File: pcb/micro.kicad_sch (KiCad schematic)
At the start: 23 parts, among them SW1 SW_Nidec_CAS-120A1, U1 ESP32-C6, Y1 7M40000049

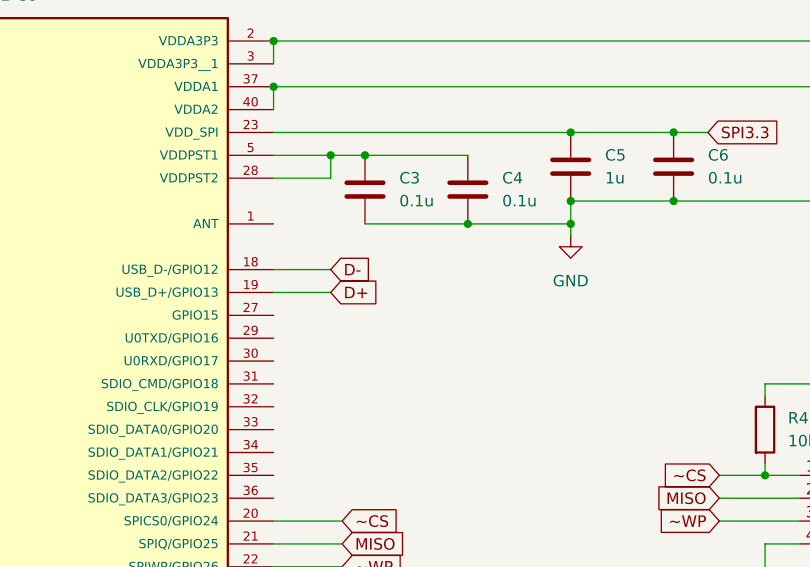
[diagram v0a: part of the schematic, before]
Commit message: Schematic finalized and general layout completed
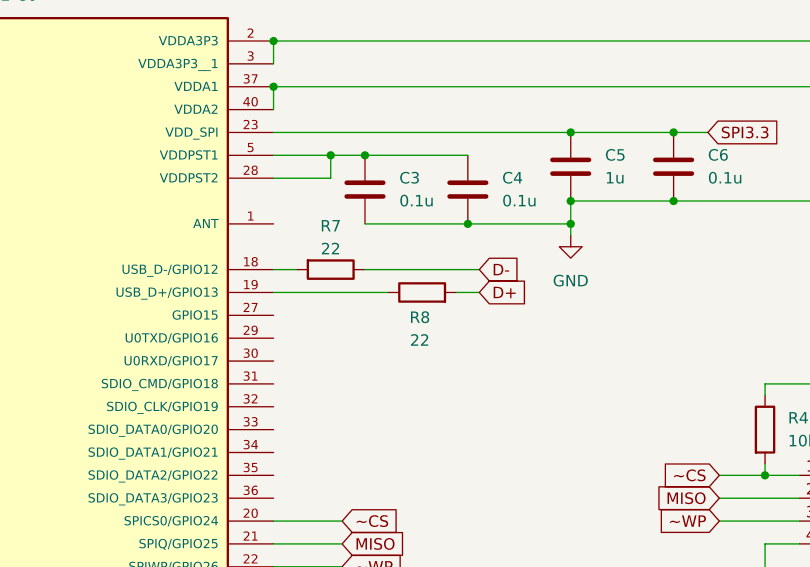
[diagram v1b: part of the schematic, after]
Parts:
- added R7, R8: 22, Resistor_SMD:R_0402_1005Metric_Pad0.72x0.64mm_HandSolder, symbol Device:R
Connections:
- net D+: now also R8.2; no longer U1.19 (USB_D+/GPIO13)
- net D-: now also R7.1; no longer U1.18 (USB_D-/GPIO12)
- new net: R7.2, U1.18 (USB_D-/GPIO12)
- new net: R8.1, U1.19 (USB_D+/GPIO13)
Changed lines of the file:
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@@
 	(wire
 		(pts
-			(xy 142.24 87.63) (xy 148.59 87.63)
+			(xy 162.56 90.17) (xy 165.1 90.17)
 		)
 		(stroke
@@
 	(wire
 		(pts
+			(xy 142.24 87.63) (xy 144.78 87.63)
+		)
+		(stroke
+			(width 0)
+			(type default)
+		)
+	)
+	(wire
+		(pts
 			(xy 54.61 115.57) (xy 54.61 120.65)
 		)
@@
 	(wire
 		(pts
-			(xy 142.24 90.17) (xy 148.59 90.17)
-		)
-		(stroke
-			(width 0)
-			(type default)
-		)
-	)
-	(wire
-		(pts
 			(xy 113.03 176.53) (xy 97.79 176.53)
 		)
@@
 	(wire
 		(pts
+			(xy 142.24 90.17) (xy 154.94 90.17)
+		)
+		(stroke
+			(width 0)
+			(type default)
+		)
+	)
+	(wire
+		(pts
 			(xy 142.24 62.23) (xy 142.24 64.77)
 		)
@@
 	(wire
 		(pts
+			(xy 152.4 87.63) (xy 165.1 87.63)
+		)
+		(stroke
+			(width 0)
+			(type default)
+		)
+	)
+	(wire
+		(pts
 			(xy 76.2 85.09) (xy 81.28 85.09)
 		)
@@
 	(global_label "D+"
 		(shape input)
-		(at 148.59 90.17 0)
+		(at 165.1 90.17 0)
 		(fields_autoplaced yes)
 		(effects
@@
 		)
 		(property "Intersheetrefs" "${INTERSHEET_REFS}"
-			(at 154.4176 90.17 0)
+			(at 170.9276 90.17 0)
 			(effects
 				(font
@@
 	(global_label "D-"
 		(shape input)
-		(at 148.59 87.63 0)
+		(at 165.1 87.63 0)
 		(fields_autoplaced yes)
 		(effects
@@
 		)
 		(property "Intersheetrefs" "${INTERSHEET_REFS}"
-			(at 154.4176 87.63 0)
+			(at 170.9276 87.63 0)
 			(effects
 				(font
@@
 	)
 	(symbol
+		(lib_id "Device:R")
+		(at 148.59 87.63 270)
+		(unit 1)
+		(exclude_from_sim no)
+		(in_bom yes)
+		(on_board yes)
+		(dnp no)
+		(property "Reference" "R7"
+			(at 148.59 82.804 90)
+			(effects
+				(font
+					(size 1.27 1.27)
+				)
+			)
+		)
+		(property "Value" "22"
+			(at 148.59 85.344 90)
+			(effects
+				(font
+					(size 1.27 1.27)
+				)
+			)
+		)
+		(property "Footprint" "Resistor_SMD:R_0402_1005Metric_Pad0.72x0.64mm_HandSolder"
+			(at 148.59 85.852 90)
+			(effects
+				(font
+					(size 1.27 1.27)
+				)
+				(hide yes)
+			)
+		)
+		(property "Datasheet" "~"
+			(at 148.59 87.63 0)
+			(effects
+				(font
+					(size 1.27 1.27)
+				)
+				(hide yes)
+			)
+		)
+		(property "Description" "Resistor"
+			(at 148.59 87.63 0)
+			(effects
+				(font
+					(size 1.27 1.27)
+				)
+				(hide yes)
+			)
+		)
+		(pin "2"
+		)
+		(pin "1"
+		)
+		(instances
+			(project "60_keyboard"
+				(path "/60f4ab9d-718b-428d-904c-5042759d3860/a5dc5d45-cfa6-4235-a666-1339e0663470"
+					(reference "R7")
+					(unit 1)
+				)
+			)
+		)
+	)
+	(symbol
 		(lib_id "Device:C")
 		(at 259.08 66.04 0)
@@
 					(unit 1)
 				)
+			)
+		)
+	)
+	(symbol
+		(lib_id "Device:R")
+		(at 158.75 90.17 90)
+		(unit 1)
+		(exclude_from_sim no)
+		(in_bom yes)
+		(on_board yes)
+		(dnp no)
+		(property "Reference" "R8"
+			(at 158.496 92.964 90)
+			(effects
+				(font
+					(size 1.27 1.27)
+				)
+			)
+		)
+		(property "Value" "22"
+			(at 158.496 95.504 90)
+			(effects
+				(font
+					(size 1.27 1.27)
+				)
+			)
+		)
+		(property "Footprint" "Resistor_SMD:R_0402_1005Metric_Pad0.72x0.64mm_HandSolder"
+			(at 158.75 91.948 90)
+			(effects
+				(font
+					(size 1.27 1.27)
+				)
+				(hide yes)
+			)
+		)
+		(property "Datasheet" "~"
+			(at 158.75 90.17 0)
+			(effects
+				(font
+					(size 1.27 1.27)
+				)
+				(hide yes)
+			)
+		)
+		(property "Description" "Resistor"
+			(at 158.75 90.17 0)
+			(effects
+				(font
+					(size 1.27 1.27)
+				)
+				(hide yes)
+			)
+		)
+		(pin "2"
+		)
+		(pin "1"
+		)
+		(instances
+			(project "60_keyboard"
+				(path "/60f4ab9d-718b-428d-904c-5042759d3860/a5dc5d45-cfa6-4235-a666-1339e0663470"
+					(reference "R8")
+					(unit 1)
+				)
